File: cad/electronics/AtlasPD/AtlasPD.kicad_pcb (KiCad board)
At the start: 4 copper layers, 150.4 x 115.3 mm, 67 parts, among them J1 Conn_01x02_Male, J2 Conn_01x02_Male, J201 USB_C_Receptacle_USB2.0, J202 Conn_01x04, J301 Conn_01x06, J302 Conn_01x06, J401 Conn_01x04, SW201 SW_SPST, U201 CP2104, U202 ATmega328P-AU, U301 74LS08, U302 DRV8837C, U303 DRV8837C, U401 AMS1117-3.3, U402 LM2678T-ADJ_NOPB, Y201 CSTNE16M0V53-R0

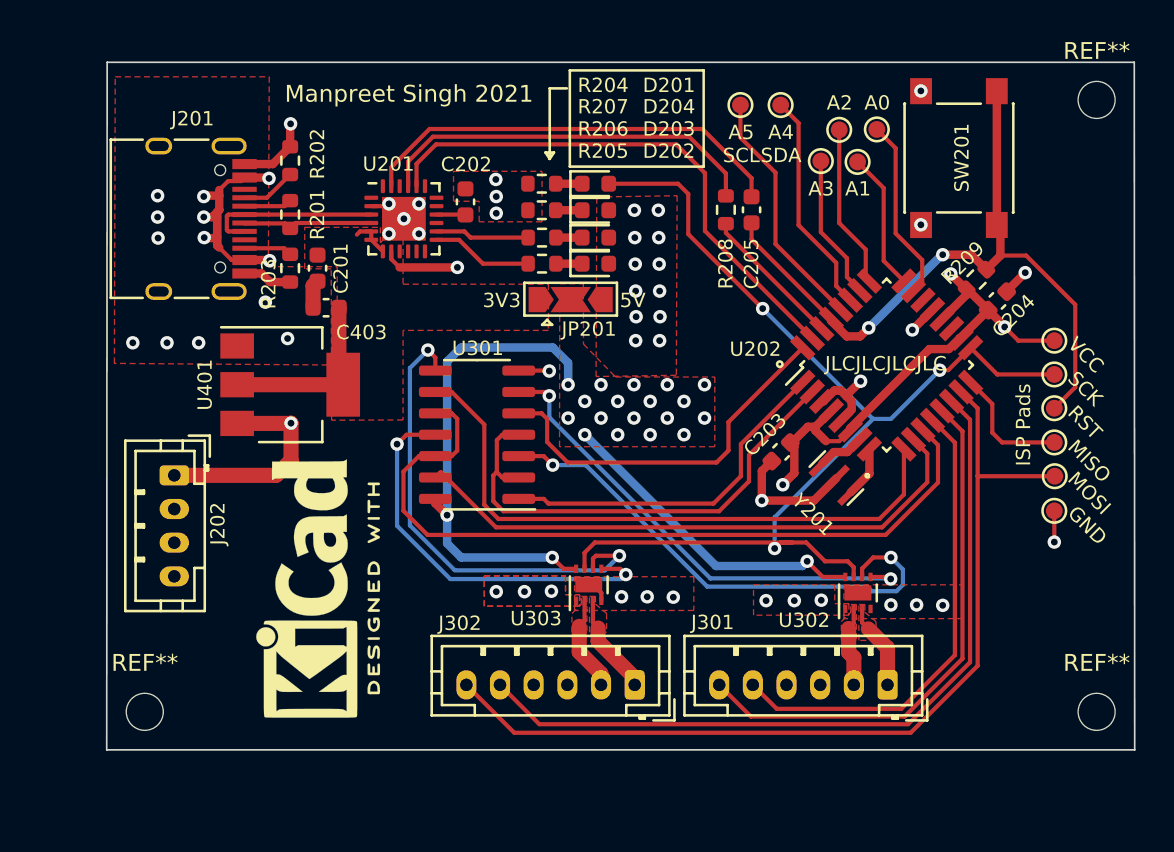
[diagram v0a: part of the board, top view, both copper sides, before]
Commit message: Getting Ready to Fab MCU
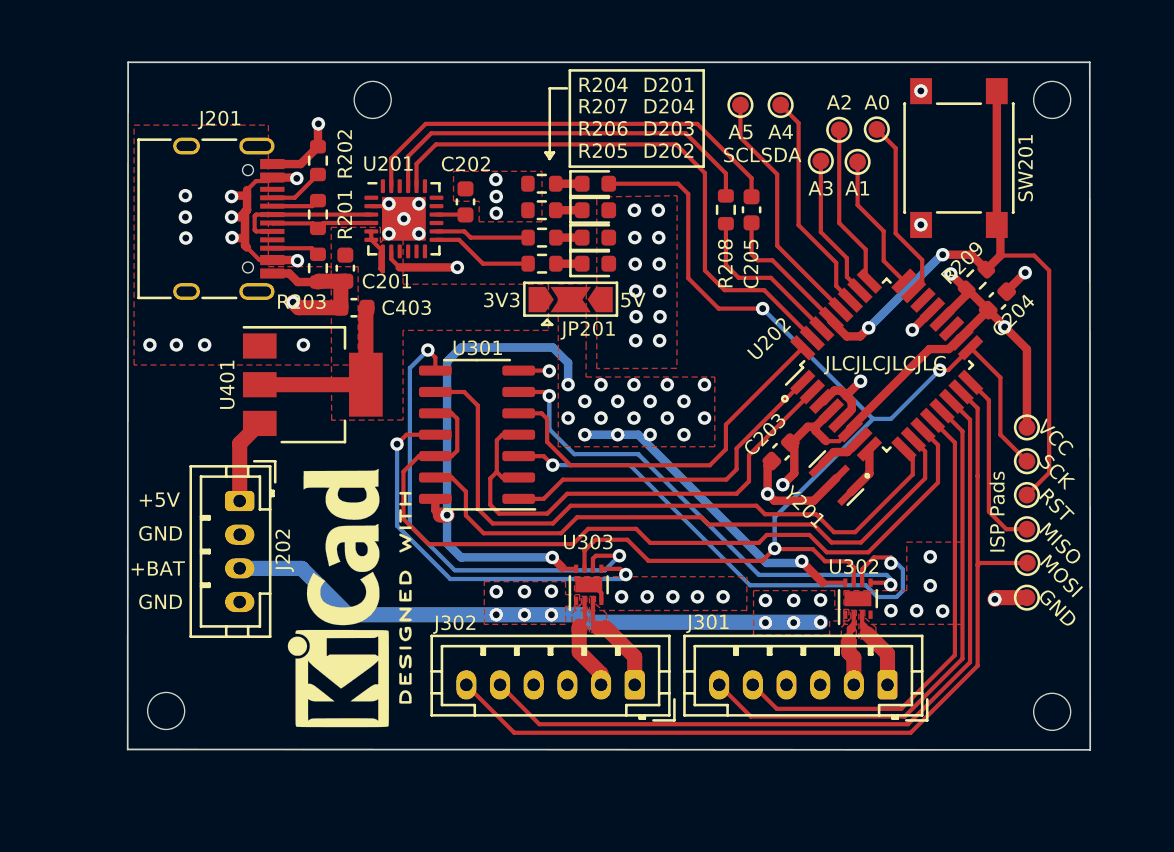
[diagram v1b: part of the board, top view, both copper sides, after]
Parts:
- added REF**: MountingHole_2.2mm_M2_DIN965, MountingHole:MountingHole_2.2mm_M2_DIN965, F.Cu at (216.3, 29.6)
- added REF**: WEEE-Logo_8.4x12mm_SilkScreen, Symbol:WEEE-Logo_8.4x12mm_SilkScreen, B.Cu at (253.4, 56.2)
- moved TP208 5.41 mm to (255.2, 53.1)
- moved TP207 5.41 mm to (255.2, 59.2)
- moved TP209 5.41 mm to (255.2, 51.1)
- moved TP210 5.41 mm to (255.2, 55.1)
- moved TP212 5.41 mm to (255.2, 49.1)
- moved TP211 5.41 mm to (255.2, 57.1)
- moved J202 4.17 mm to (208.4, 53.5)
- moved REF** 2.64 mm to (256.7, 66.0)
- moved REF** 2.64 mm to (256.7, 29.6)
- moved REF** 1.96 mm to (214.2, 59.2)
- moved C201 1.65 mm to (214.7, 39.6)
- moved J201 1.65 mm to (206.3, 36.7)
- moved R201 1.65 mm to (213.1, 36.4)
- moved R202 1.65 mm to (213.1, 33.2)
- moved R203 1.65 mm to (213.1, 39.6)
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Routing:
- net +BATT: track 0.00 -> 35.8 mm, vias 6 -> 12
- net +5V: track 90.8 -> 79.0 mm, vias 19 -> 18
- net /Sheet60A2E58A/RESET: track 43.2 -> 48.7 mm
- net /Motor Driver/EN: track 65.7 -> 69.8 mm
- net GND: track 34.8 -> 38.8 mm, vias 65 -> 69
- net VCC: track 79.6 -> 83.1 mm
- net /Sheet60A2E58A/IO12_MISO: track 7.45 -> 10.8 mm
- net /Motor Driver/IN3: track 37.1 -> 39.4 mm
- net /Motor Driver/PWM_B: track 46.5 -> 48.8 mm
- net /Motor Driver/IN4: track 34.7 -> 36.5 mm
- net /Sheet60A2E58A/USB_DN: track 7.80 -> 6.15 mm
- net /Motor Driver/S4: track 54.5 -> 52.9 mm
- net +3V3: track 13.4 -> 14.9 mm
- net /Sheet60A2E58A/IO1: track 32.1 -> 33.5 mm
- net /Sheet60A2E58A/IO0: track 8.60 -> 9.72 mm
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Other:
- board size 150.4 x 115.3 mm -> 147.8 x 115.3 mm
- rule trace_min: 0.2 -> 0
- board text added: "+BAT"
- board text added: "Atlas MCU Rev. 1.0"
